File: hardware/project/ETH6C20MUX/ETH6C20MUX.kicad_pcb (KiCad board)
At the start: 4 copper layers, 160 x 100 mm, 197 parts, among them J301 5499141-4, J501 Conn_02x06_Odd_Even, J502 Conn_02x08_Odd_Even, J503 C64AC, J601 Conn_02x05, J602 Conn_02x01, K301 HE3621A0510, K302 HE3621A0510, K303 HE3621A0510, K304 HE3621A0510, K305 HE3621A0510, K306 HE3621A0510, K307 HE3621A0510, K308 HE3621A0510, K309 HE3621A0510, K310 HE3621A0510, K311 HE3621A0510, K312 HE3621A0510, K313 HE3621A0510, K314 HE3621A0510, K315 HE3621A0510, K316 HE3621A0510, K317 HE3621A0510, K318 HE3621A0510, K319 HE3621A0510, K320 HE3621A0510, K321 HE3621A0510, K322 HE3621A0510, K323 HE3621A0510, K324 HE3621A0510, K325 HE3621A0510, K326 HE3621A0510, K327 HE3621A0510, K328 HE3621A0510, K329 HE3621A0510, K330 HE3621A0510, K331 HE3621A0510, K332 HE3621A0510, K333 HE3621A0510, K334 HE3621A0510, K335 HE3621A0510, K336 HE3621A0510, K337 HE3621A0510, K338 HE3621A0510, K339 HE3621A0510, K340 HE3621A0510, K341 HE3621A0510, K342 HE3621A0510, K343 HE3621A0510, K344 HE3621A0510, K345 HE3621A0510, K346 HE3621A0510, K347 HE3621A0510, K348 HE3621A0510, K349 HE3621A0510, K350 HE3621A0510, K351 HE3621A0510, K352 HE3621A0510, K353 HE3621A0510, K354 HE3621A0510, K355 HE3621A0510, K356 HE3621A0510, K357 HE3621A0510, K358 HE3621A0510, K359 HE3621A0510, K360 HE3621A0510, K361 HE3621A0510, K362 HE3621A0510, K363 HE3621A0510, K364 HE3621A0510, K365 HE3621A0510, K366 HE3621A0510, K367 HE3621A0510, K368 HE3621A0510, K369 HE3621A0510, K370 HE3621A0510, Q401 IRFR5410, SW601 A6SN-5104, U201 LC03-3.3, U202 LAN8742A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

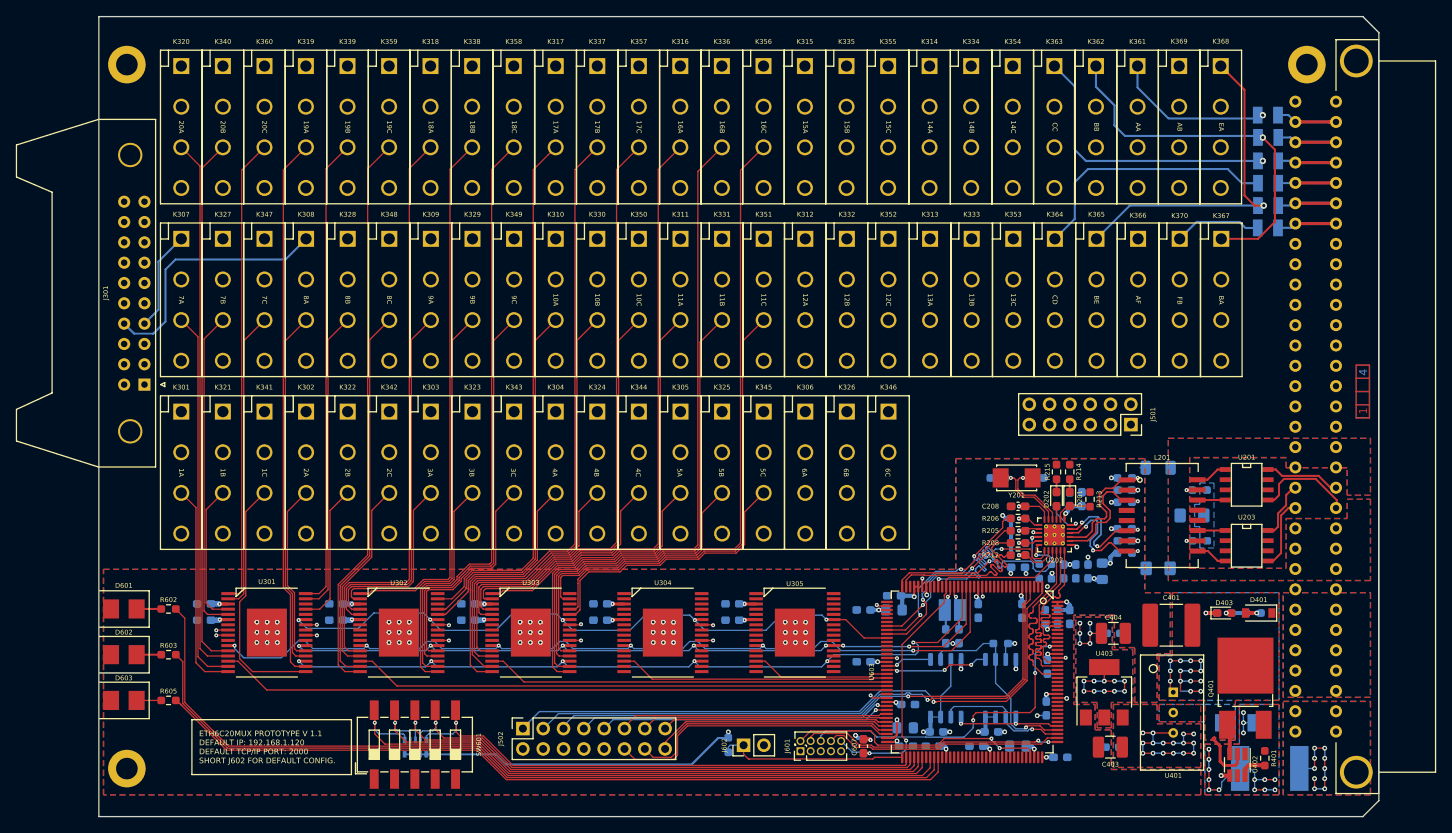
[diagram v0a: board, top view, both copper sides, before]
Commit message: Main PCB layout done
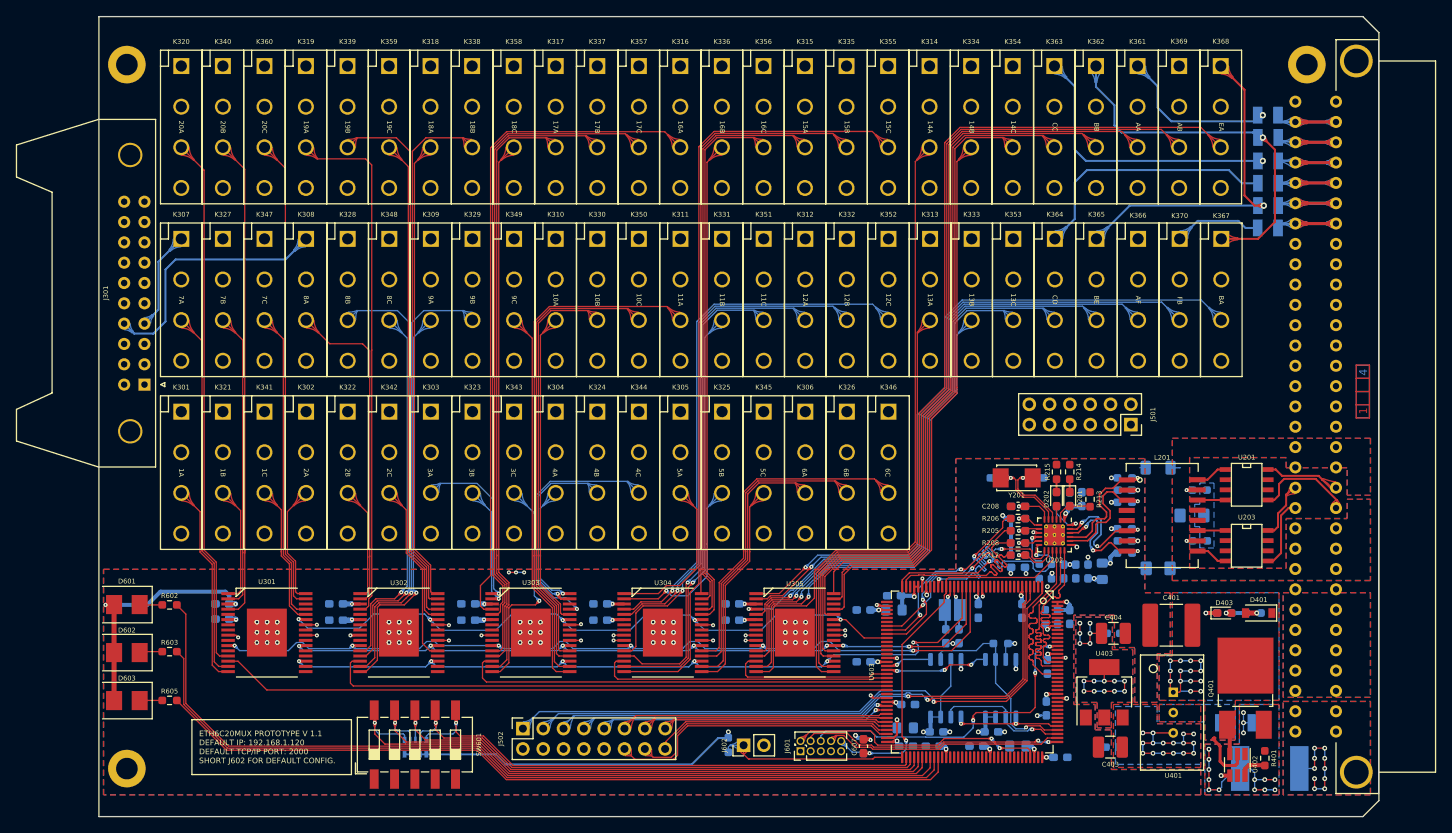
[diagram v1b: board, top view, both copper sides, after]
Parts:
- moved C306 2.29 mm to (75.4, 115.3)
- moved C301 2.29 mm to (75.4, 113.4)
- moved D601 0.67 mm to (63.5, 113.5)
- moved R602 0.52 mm to (68.8, 113.5)
- moved D602 0.46 mm to (63.5, 119.5)
- moved R603 0.40 mm to (68.8, 119.4)
- moved D603 0.38 mm to (63.5, 125.5)
- moved R605 0.13 mm to (68.8, 125.5)
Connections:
- K315 pad 3: (no net) -> /Relays/RELAY15A
- K335 pad 3: (no net) -> /Relays/RELAY15B
- K354 pad 3: (no net) -> /Relays/RELAY14C
- K355 pad 3: (no net) -> /Relays/RELAY15C
- U301 pad 1: /Relays/RELAY20C -> /Relays/RELAY1B
- U301 pad 12: /Relays/RELAY20B -> (no net)
- U301 pad 17: /Relays/RELAY1C -> (no net)
- U301 pad 18: /Relays/RELAY19A -> (no net)
- U301 pad 2: /Relays/RELAY7C -> /Relays/RELAY7B
- U301 pad 20: /Relays/RELAY8A -> (no net)
- U301 pad 21: /Relays/RELAY2A -> (no net)
- U301 pad 28: (no net) -> /Relays/RELAY1C
- U301 pad 29: /Relays/RELAY2B -> /Relays/RELAY7C
- U301 pad 31: /Relays/RELAY8B -> /Relays/RELAY20C
- U301 pad 32: /Relays/RELAY19B -> /Relays/RELAY2A
- U301 pad 4: /Relays/RELAY1B -> /Relays/RELAY20B
- U301 pad 5: /Relays/RELAY7B -> (no net)
- U302 pad 1: /Relays/RELAY9B -> /Relays/RELAY2B
- U302 pad 12: /Relays/RELAY18A -> /Relays/RELAY8C
- U302 pad 13: /Relays/RELAY2C -> /Relays/RELAY8B
- U302 pad 15: /Relays/RELAY8C -> /Relays/RELAY9B
- U302 pad 16: /Relays/RELAY19C -> /Relays/RELAY9A
- U302 pad 17: /Relays/RELAY3B -> (no net)
- U302 pad 18: /Relays/RELAY18C -> (no net)
- U302 pad 2: /Relays/RELAY18B -> /Relays/RELAY8A
- U302 pad 20: /Relays/RELAY9C -> (no net)
- U302 pad 21: /Relays/RELAY3C -> /Relays/RELAY2C
- U302 pad 28: /Relays/RELAY4A -> /Relays/RELAY19C
- U302 pad 29: /Relays/RELAY10A -> /Relays/RELAY19B
- U302 pad 31: /Relays/RELAY17A -> /Relays/RELAY18B
- U302 pad 32: (no net) -> /Relays/RELAY18A
- U302 pad 4: /Relays/RELAY3A -> /Relays/RELAY19A
- U302 pad 5: /Relays/RELAY9A -> (no net)
- U303 pad 1: /Relays/RELAY11A -> /Relays/RELAY3A
- U303 pad 12: /Relays/RELAY17C -> /Relays/RELAY17B
- U303 pad 13: /Relays/RELAY4B -> /Relays/RELAY17A
- U303 pad 15: /Relays/RELAY10B -> /Relays/RELAY18C
- U303 pad 16: /Relays/RELAY17B -> /Relays/RELAY3C
- U303 pad 17: /Relays/RELAY5A -> /Relays/RELAY9C
- U303 pad 18: /Relays/RELAY16B -> /Relays/RELAY11A
- U303 pad 2: /Relays/RELAY16A -> /Relays/RELAY3B
- U303 pad 20: /Relays/RELAY11B -> /Relays/RELAY10C
- U303 pad 21: /Relays/RELAY5B -> /Relays/RELAY10B
- U303 pad 28: /Relays/RELAY5C -> /Relays/RELAY10A
- U303 pad 29: /Relays/RELAY11C -> /Relays/RELAY4C
- U303 pad 31: /Relays/RELAY16C -> /Relays/RELAY4B
- U303 pad 32: (no net) -> /Relays/RELAY4A
- U303 pad 4: /Relays/RELAY4C -> /Relays/RELAY16A
- U303 pad 5: /Relays/RELAY10C -> /Relays/RELAY17C
- U304 pad 1: (no net) -> /Relays/RELAY5A
- U304 pad 12: (no net) -> /Relays/RELAY12A
- U304 pad 13: (no net) -> /Relays/RELAY11C
- U304 pad 15: (no net) -> /Relays/RELAY11B
- U304 pad 16: (no net) -> /Relays/RELAY15C
- U304 pad 17: (no net) -> /Relays/RELAY5C
- U304 pad 18: /Relays/RELAY12A -> /Relays/RELAY6A
- U304 pad 2: (no net) -> /Relays/RELAY5B
- U304 pad 20: /Relays/RELAY12B -> /Relays/RELAY6B
- U304 pad 21: /Relays/RELAY12C -> /Relays/RELAY6C
- U304 pad 28: /Relays/RELAY6A -> /Relays/RELAY16B
- U304 pad 29: /Relays/RELAY6B -> /Relays/RELAY16C
- U304 pad 31: /Relays/RELAY6C -> /Relays/RELAY15A
- U304 pad 32: (no net) -> /Relays/RELAY15B
- U304 pad 4: (no net) -> /Relays/RELAY12C
- U304 pad 5: (no net) -> /Relays/RELAY12B
- U305 pad 1: /Relays/RELAY14A -> /Relays/RELAYBA
- U305 pad 12: /Relays/RELAY13B -> /Relays/RELAYD
- U305 pad 15: /Relays/RELAYBA -> /Relays/RELAY13B
- U305 pad 16: /Relays/RELAYEA -> /Relays/RELAY14A
- U305 pad 17: /Relays/RELAYAB -> /Relays/RELAY13A
- U305 pad 18: /Relays/RELAYF -> /Relays/RELAYEA
- U305 pad 2: /Relays/RELAY14B -> /Relays/RELAYFA
- U305 pad 20: /Relays/RELAYE -> /Relays/RELAYAB
- U305 pad 21: /Relays/RELAYD -> /Relays/RELAYA
- U305 pad 28: /Relays/RELAYC -> /Relays/RELAYB
- U305 pad 29: /Relays/RELAYB -> /Relays/RELAY14B
- U305 pad 31: /Relays/RELAYA -> /Relays/RELAY14C
- U305 pad 32: /Relays/RELAYFA -> /Relays/RELAYC
- U305 pad 4: (no net) -> /Relays/RELAYF
- U305 pad 5: /Relays/RELAY13A -> /Relays/RELAYE
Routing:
- net /Relays/RELAYEA: track 0.00 -> 115.1 mm
- net /Relays/RELAYAB: track 0.00 -> 107.9 mm
- net /Relays/RELAYA: track 0.00 -> 101.3 mm
- net /Relays/RELAY15C: track 0.00 -> 98.7 mm
- net /Relays/RELAYB: track 0.00 -> 90.8 mm
- net /Relays/RELAYBA: track 0.00 -> 89.1 mm, vias 0 -> 1
- net /Relays/RELAYFA: track 0.00 -> 84.0 mm, vias 0 -> 1
- net /Relays/RELAY14A: track 0.00 -> 83.0 mm
- net /Relays/RELAYF: track 0.00 -> 81.1 mm, vias 0 -> 1
- net /Relays/RELAYC: track 0.13 -> 81.1 mm
- net /Relays/RELAY14C: track 0.00 -> 76.0 mm
- net /Relays/RELAY15B: track 0.00 -> 75.4 mm
- net /Relays/RELAYE: track 0.00 -> 74.5 mm, vias 0 -> 1
- net /Relays/RELAYD: track 0.00 -> 74.0 mm, vias 0 -> 1
- net /Relays/RELAY15A: track 0.00 -> 71.5 mm
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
